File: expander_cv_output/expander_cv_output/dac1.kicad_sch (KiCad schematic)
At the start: 32 parts, among them U3 TL074, U4 MCP4728, U5 TL074

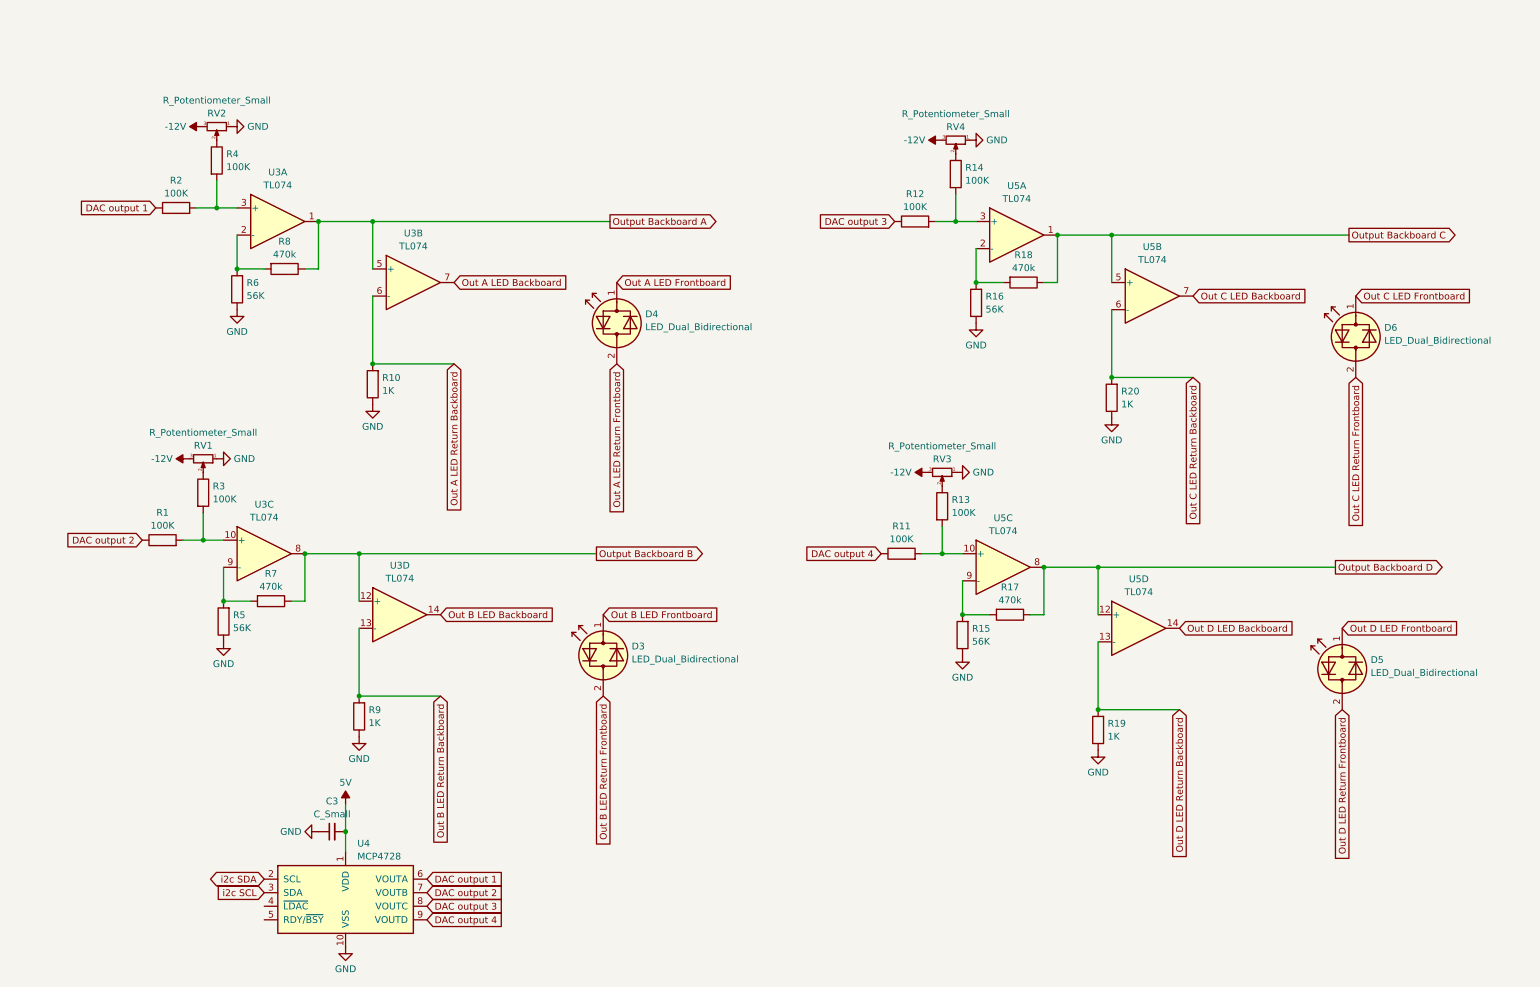
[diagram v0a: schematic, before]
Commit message: tracked first draft of expander_cv_output
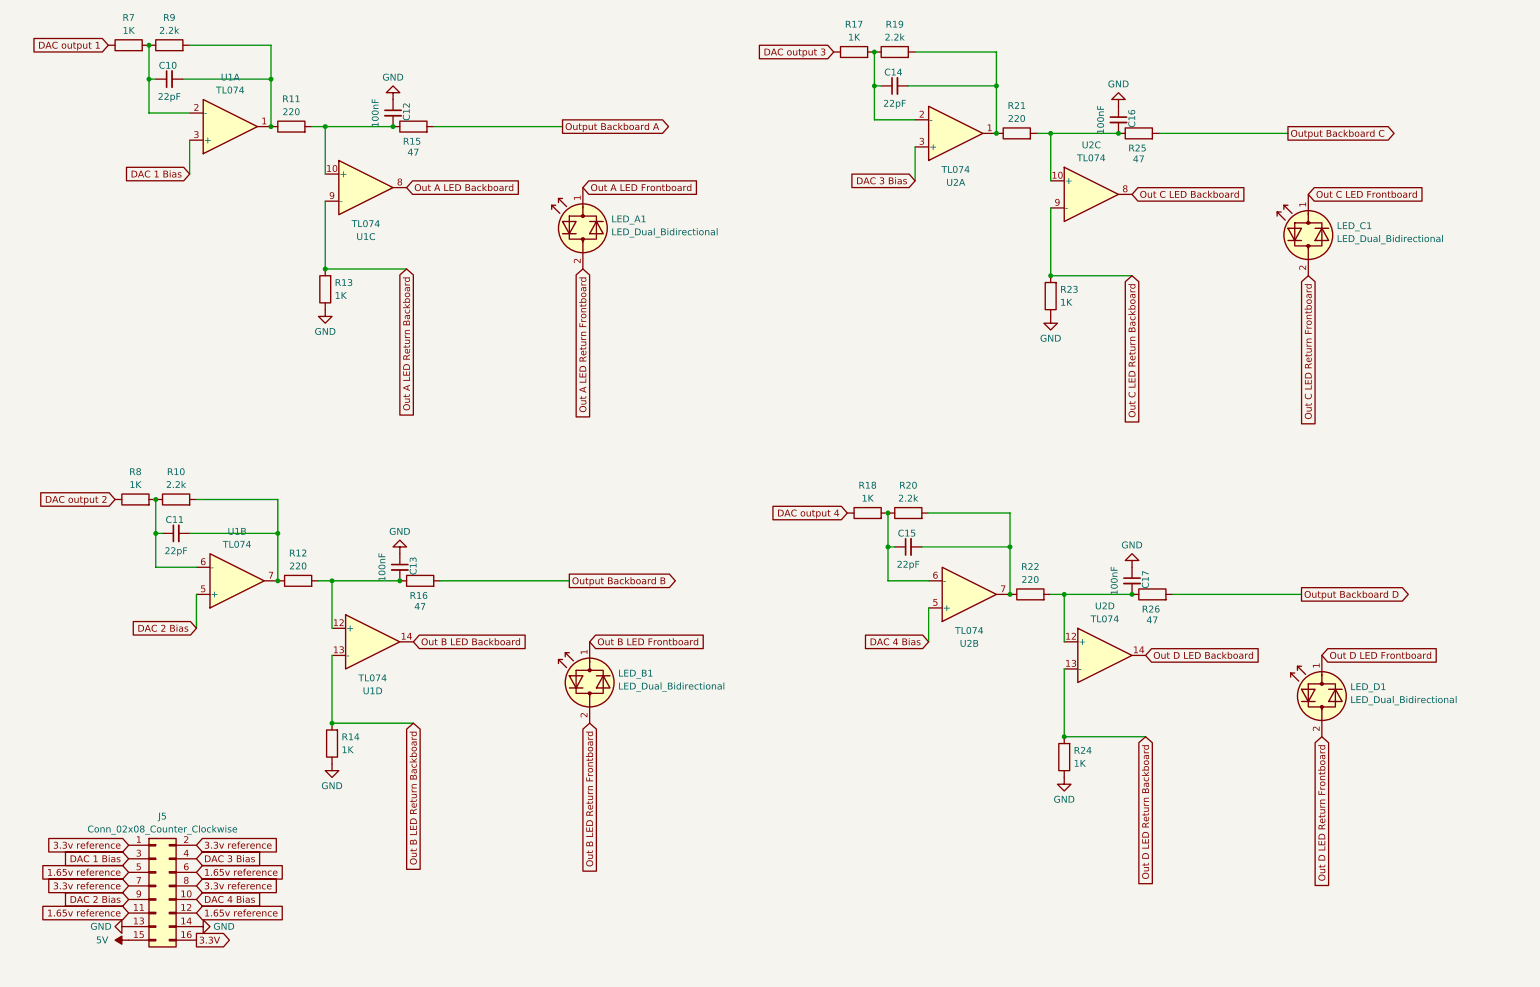
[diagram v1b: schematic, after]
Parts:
- removed C3: C_Small, Capacitor_SMD:C_0805_2012Metric_Pad1.18x1.45mm_HandSolder, symbol Device:C_Small
- removed D3, D5, D6: LED_Dual_Bidirectional, LED_THT:LED_D3.0mm, symbol Device:LED_Dual_Bidirectional
- removed R1, R13, R3, R4: 100K, Resistor_SMD:R_0603_1608Metric_Pad0.98x0.95mm_HandSolder, symbol Device:R
- removed R5, R6: 56K, Resistor_SMD:R_0603_1608Metric_Pad0.98x0.95mm_HandSolder, symbol Device:R
- removed R7: 470k, Resistor_SMD:R_0603_1608Metric_Pad0.98x0.95mm_HandSolder, symbol Device:R
- removed RV1, RV2, RV3, RV4: R_Potentiometer_Small, Potentiometer_THT:Potentiometer_Bourns_3296X_Horizontal, symbol Device:R_Potentiometer_Small
- removed U3, U5: TL074, Package_SO:TSSOP-14_4.4x5mm_P0.65mm, symbol Amplifier_Operational:TL074
- removed U4: MCP4728, Package_SO:MSOP-10_3x3mm_P0.5mm, symbol Analog_DAC:MCP4728
- added C10, C11, C14, C15: 22pF, Capacitor_SMD:C_0805_2012Metric_Pad1.18x1.45mm_HandSolder, symbol Device:C_Small
- added C12, C13, C16, C17: 100nF, Capacitor_SMD:C_0805_2012Metric_Pad1.18x1.45mm_HandSolder, symbol Device:C_Small
- added J5: Conn_02x08_Counter_Clockwise, Connector_PinHeader_2.54mm:PinHeader_2x08_P2.54mm_Vertical, symbol Connector_Generic:Conn_02x08_Odd_Even
- added LED_B1, LED_C1, LED_D1: LED_Dual_Bidirectional, LED_THT:LED_D3.0mm, symbol Device:LED_Dual_Bidirectional
- added R10: 2.2k, Resistor_SMD:R_0805_2012Metric_Pad1.20x1.40mm_HandSolder, symbol Device:R
- added R21, R22: 220, Resistor_SMD:R_0805_2012Metric_Pad1.20x1.40mm_HandSolder, symbol Device:R
- added R23, R24: 1K, Resistor_SMD:R_0805_2012Metric_Pad1.20x1.40mm_HandSolder, symbol Device:R
- added R25, R26: 47, Resistor_SMD:R_0805_2012Metric_Pad1.20x1.40mm_HandSolder, symbol Device:R
- added U1, U2: TL074, Package_SO:SOIC-14_3.9x8.7mm_P1.27mm, symbol Amplifier_Operational:TL074
- R11, R12: value 100K -> 220; footprint Resistor_SMD:R_0603_1608Metric_Pad0.98x0.95mm_HandSolder -> Resistor_SMD:R_0805_2012Metric_Pad1.20x1.40mm_HandSolder
- R13: renamed from R10; footprint Resistor_SMD:R_0603_1608Metric_Pad0.98x0.95mm_HandSolder -> Resistor_SMD:R_0805_2012Metric_Pad1.20x1.40mm_HandSolder
- R14: value 100K -> 1K; footprint Resistor_SMD:R_0603_1608Metric_Pad0.98x0.95mm_HandSolder -> Resistor_SMD:R_0805_2012Metric_Pad1.20x1.40mm_HandSolder
- R15, R16: value 56K -> 47; footprint Resistor_SMD:R_0603_1608Metric_Pad0.98x0.95mm_HandSolder -> Resistor_SMD:R_0805_2012Metric_Pad1.20x1.40mm_HandSolder
- R17, R18, R8: value 470k -> 1K; footprint Resistor_SMD:R_0603_1608Metric_Pad0.98x0.95mm_HandSolder -> Resistor_SMD:R_0805_2012Metric_Pad1.20x1.40mm_HandSolder
- R19, R20, R9: value 1K -> 2.2k; footprint Resistor_SMD:R_0603_1608Metric_Pad0.98x0.95mm_HandSolder -> Resistor_SMD:R_0805_2012Metric_Pad1.20x1.40mm_HandSolder
- R7: renamed from R2; value 100K -> 1K; footprint Resistor_SMD:R_0603_1608Metric_Pad0.98x0.95mm_HandSolder -> Resistor_SMD:R_0805_2012Metric_Pad1.20x1.40mm_HandSolder
- renumbered D4 to LED_A1
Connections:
- net 5V: now also J5.15 (Pin_15)
- net DAC output 2: now also R8.1
- net DAC output 3: now also R17.1; no longer R12.1
- net DAC output 4: now also R18.1; no longer R11.1
- net GND: now also R14.1, C12.1, C13.1, C16.1, C17.1, J5.13 (Pin_13), J5.14 (Pin_14), R23.1, R24.1; no longer R15.1, R16.1, R19.1, R20.1, R9.1
- net Out A LED Backboard: now also U1.8
- net Out A LED Return Backboard: now also U1.9 (-)
- net Out B LED Backboard: now also U1.14
- net Out B LED Frontboard: now also LED_B1.1 (KA)
- net Out B LED Return Backboard: now also R14.2, U1.13 (-); no longer R9.2
- net Out B LED Return Frontboard: now also LED_B1.2 (AK)
- net Out C LED Backboard: now also U2.8
- net Out C LED Frontboard: now also LED_C1.1 (KA)
- net Out C LED Return Backboard: now also R23.2, U2.9 (-); no longer R20.2
- net Out C LED Return Frontboard: now also LED_C1.2 (AK)
- net Out D LED Backboard: now also U2.14
- net Out D LED Frontboard: now also LED_D1.1 (KA)
- net Out D LED Return Backboard: now also R24.2, U2.13 (-); no longer R19.2
- net Out D LED Return Frontboard: now also LED_D1.2 (AK)
- net Output Backboard A: now also R15.2; no longer R8.1
- net Output Backboard B: now also R16.2
- net Output Backboard C: now also R25.2; no longer R18.1
- net Output Backboard D: now also R26.2; no longer R17.1
- net at R17.2: now also R19.1, C14.1, U2.2 (-); no longer R15.2
- net at R12.2: now also R16.1, C13.2, U1.12 (+); no longer R14.2
- net at R11.2: now also R15.1, C12.2, U1.10 (+)
- net at R18.2: now also R20.1, C15.1, U2.6 (-); no longer R16.2
- net at R8.2: now also C11.1, R10.1, U1.6 (-)
- net at R7.2: now also R9.1, C10.1, U1.2 (-)
- new net: C16.2, R21.2, R25.1, U2.10 (+)
- new net: C15.2, R20.2, R22.1, U2.7
- new net: C14.2, R19.2, R21.1, U2.1
- new net: C10.2, R11.1, R9.2, U1.1
- new net: C11.2, R10.2, R12.1, U1.7
- new net: C17.2, R22.2, R26.1, U2.12 (+)
- new net 1.65v reference: J5.11 (Pin_11), J5.12 (Pin_12), J5.5 (Pin_5), J5.6 (Pin_6)
- new net 3.3V: J5.16 (Pin_16)
- new net 3.3v reference: J5.1 (Pin_1), J5.2 (Pin_2), J5.7 (Pin_7), J5.8 (Pin_8)
- new net DAC 1 Bias: J5.3 (Pin_3), U1.3 (+)
- new net DAC 2 Bias: J5.9 (Pin_9), U1.5 (+)
- new net DAC 3 Bias: J5.4 (Pin_4), U2.3 (+)
- new net DAC 4 Bias: J5.10 (Pin_10), U2.5 (+)
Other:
- moved on the sheet: LED_A1, R13, R7
